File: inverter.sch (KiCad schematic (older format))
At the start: 23 parts, among them P1 CONN_01X02, P2 CONN_01X02, P3 CONN_01X02, U1 LM25576MH

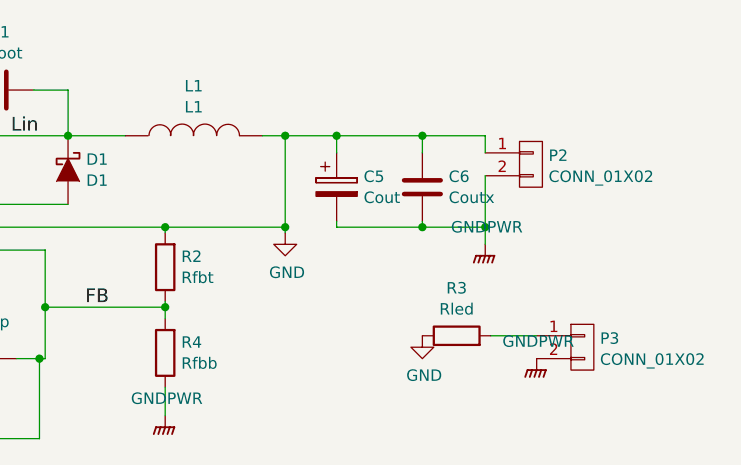
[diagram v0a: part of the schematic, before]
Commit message: Fertig gestellt
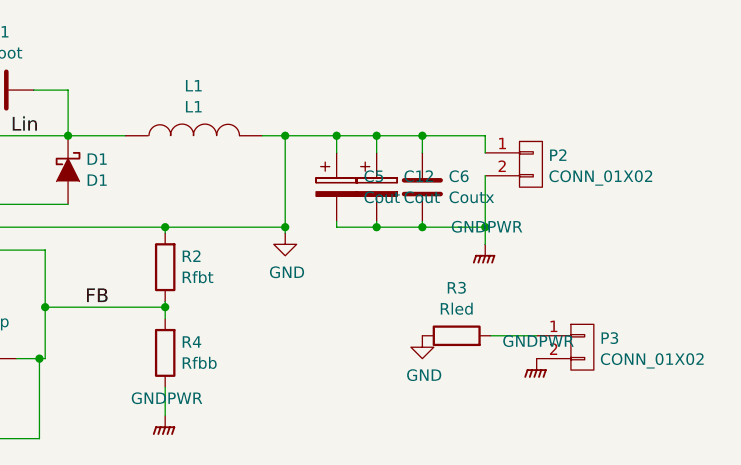
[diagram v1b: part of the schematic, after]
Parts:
- added C12: Cout, Capacitors_Tantalum_SMD:TantalC_SizeB_EIA-3528_Reflow, symbol CP
- C5: footprint Capacitors_ThroughHole:C_Radial_D6.3_L11.2_P2.5 -> Capacitors_Tantalum_SMD:TantalC_SizeB_EIA-3528_Reflow
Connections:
- net GND: now also C12.1
- net GNDPWR: now also C12.2
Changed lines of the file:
@@
 LIBS:valves
 LIBS:Special
+LIBS:inverter-cache
 EELAYER 25 0
 EELAYER END
@@
 $EndComp
 $Comp
-L GNDPWR #PWR01
+L GNDPWR #PWR10
 U 1 1 56AF6ED5
 P 5475 4100
-F 0 "#PWR01" H 5475 3900 50  0001 C CNN
+F 0 "#PWR10" H 5475 3900 50  0001 C CNN
 F 1 "GNDPWR" H 5482 4175 50  0000 C CNN
 F 2 "" H 5475 4050 50  0000 C CNN
@@
 $EndComp
 $Comp
-L GND #PWR02
+L GND #PWR2
 U 1 1 56AF7015
 P 2475 2900
-F 0 "#PWR02" H 2475 2650 50  0001 C CNN
+F 0 "#PWR2" H 2475 2650 50  0001 C CNN
 F 1 "GND" H 2483 2726 50  0000 C CNN
 F 2 "" H 2475 2900 50  0000 C CNN
@@
 Connection ~ 3225 2825
 $Comp
-L GND #PWR03
+L GND #PWR5
 U 1 1 56AF7176
 P 2925 3225
-F 0 "#PWR03" H 2925 2975 50  0001 C CNN
+F 0 "#PWR5" H 2925 2975 50  0001 C CNN
 F 1 "GND" H 2933 3051 50  0000 C CNN
 F 2 "" H 2925 3225 50  0000 C CNN
@@
 $EndComp
 $Comp
-L GND #PWR04
+L GND #PWR3
 U 1 1 56AF71A3
 P 3225 3200
-F 0 "#PWR04" H 3225 2950 50  0001 C CNN
+F 0 "#PWR3" H 3225 2950 50  0001 C CNN
 F 1 "GND" H 3233 3026 50  0000 C CNN
 F 2 "" H 3225 3200 50  0000 C CNN
@@
 $EndComp
 $Comp
-L GNDPWR #PWR05
+L GNDPWR #PWR4
 U 1 1 56AF7472
 P 3625 3200
-F 0 "#PWR05" H 3625 3000 50  0001 C CNN
+F 0 "#PWR4" H 3625 3000 50  0001 C CNN
 F 1 "GNDPWR" H 3632 3275 50  0000 C CNN
 F 2 "" H 3625 3150 50  0000 C CNN
@@
 Connection ~ 4725 4125
 $Comp
-L GNDPWR #PWR06
+L GNDPWR #PWR12
 U 1 1 56AF7AAE
 P 4725 4200
-F 0 "#PWR06" H 4725 4000 50  0001 C CNN
+F 0 "#PWR12" H 4725 4000 50  0001 C CNN
 F 1 "GNDPWR" H 4732 4275 50  0000 C CNN
 F 2 "" H 4725 4150 50  0000 C CNN
@@
 $EndComp
 $Comp
-L GNDPWR #PWR07
+L GNDPWR #PWR7
 U 1 1 56AF8416
 P 8600 3400
-F 0 "#PWR07" H 8600 3200 50  0001 C CNN
+F 0 "#PWR7" H 8600 3200 50  0001 C CNN
 F 1 "GNDPWR" H 8607 3475 50  0000 C CNN
 F 2 "" H 8600 3350 50  0000 C CNN
@@
 F 0 "C5" H 8068 3196 50  0000 L CNN
 F 1 "Cout" H 8068 3104 50  0000 L CNN
-F 2 "Capacitors_ThroughHole:C_Radial_D6.3_L11.2_P2.5" H 7988 3000 50  0001 C CNN
+F 2 "Capacitors_Tantalum_SMD:TantalC_SizeB_EIA-3528_Reflow" H 7988 3000 50  0001 C CNN
 F 3 "" H 7950 3150 50  0000 C CNN
 	1    7950 3150
@@
 $EndComp
 $Comp
-L GND #PWR08
+L GND #PWR6
 U 1 1 56AF883A
 P 7725 3350
-F 0 "#PWR08" H 7725 3100 50  0001 C CNN
+F 0 "#PWR6" H 7725 3100 50  0001 C CNN
 F 1 "GND" H 7733 3176 50  0000 C CNN
 F 2 "" H 7725 3350 50  0000 C CNN
@@
 	7200 3650 7200 3725
 $Comp
-L GNDPWR #PWR09
+L GNDPWR #PWR11
 U 1 1 56AF9168
 P 7200 4150
-F 0 "#PWR09" H 7200 3950 50  0001 C CNN
+F 0 "#PWR11" H 7200 3950 50  0001 C CNN
 F 1 "GNDPWR" H 7207 4225 50  0000 C CNN
 F 2 "" H 7200 4100 50  0000 C CNN
@@
 Lin
 $Comp
-L VCC #PWR010
+L VCC #PWR1
 U 1 1 56AF9BDE
 P 2925 2725
-F 0 "#PWR010" H 2925 2575 50  0001 C CNN
+F 0 "#PWR1" H 2925 2575 50  0001 C CNN
 F 1 "VCC" H 2945 2899 50  0000 C CNN
 F 2 "" H 2925 2725 50  0000 C CNN
@@
 $EndComp
 $Comp
-L GNDPWR #PWR011
+L GNDPWR #PWR9
 U 1 1 56AFA023
 P 8825 3900
-F 0 "#PWR011" H 8825 3700 50  0001 C CNN
+F 0 "#PWR9" H 8825 3700 50  0001 C CNN
 F 1 "GNDPWR" H 8832 3975 50  0000 C CNN
 F 2 "" H 8825 3850 50  0000 C CNN
@@
 $EndComp
 $Comp
-L GND #PWR012
+L GND #PWR8
 U 1 1 56AFA09C
 P 8325 3800
-F 0 "#PWR012" H 8325 3550 50  0001 C CNN
+F 0 "#PWR8" H 8325 3550 50  0001 C CNN
 F 1 "GND" H 8333 3626 50  0000 C CNN
 F 2 "" H 8325 3800 50  0000 C CNN
@@
 Wire Wire Line
 	8625 3800 8825 3800
+$Comp
+L CP C12
+U 1 1 56B44D44
+P 8125 3150
+F 0 "C12" H 8243 3196 50  0000 L CNN
+F 1 "Cout" H 8243 3104 50  0000 L CNN
+F 2 "Capacitors_Tantalum_SMD:TantalC_SizeB_EIA-3528_Reflow" H 8163 3000 50  0001 C CNN
+F 3 "" H 8125 3150 50  0000 C CNN
+	1    8125 3150
+	1    0    0    -1
+$EndComp
+Wire Wire Line
+	8125 3300 8125 3325
+Connection ~ 8125 3325
+Wire Wire Line
+	8125 3000 8125 2925
+Connection ~ 8125 2925
 $EndSCHEMATC
